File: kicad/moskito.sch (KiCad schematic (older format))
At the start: 0 parts

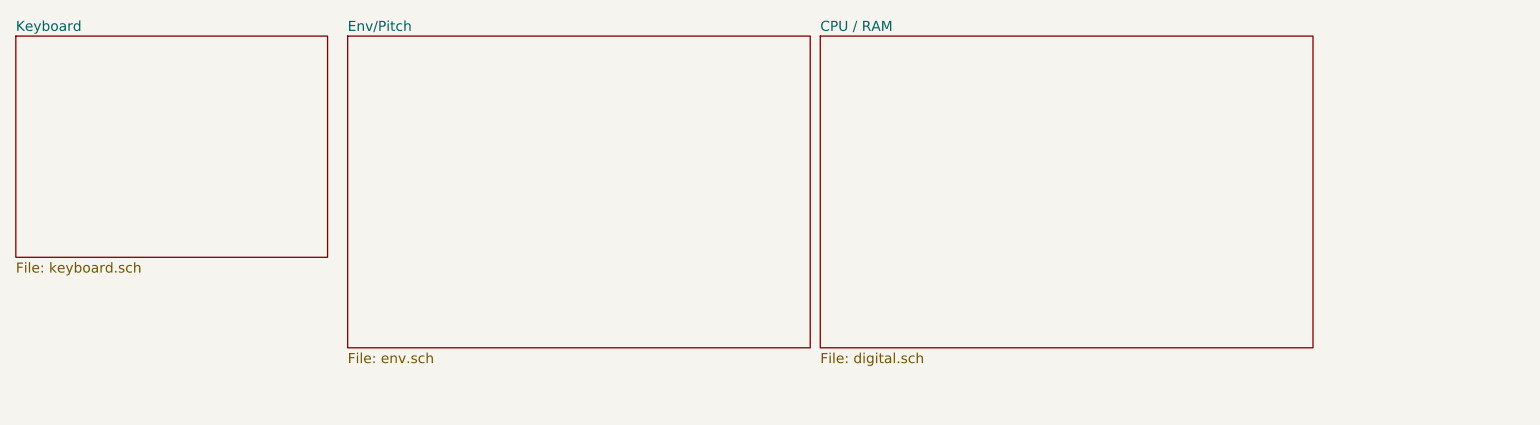
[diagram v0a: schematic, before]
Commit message: 'a'
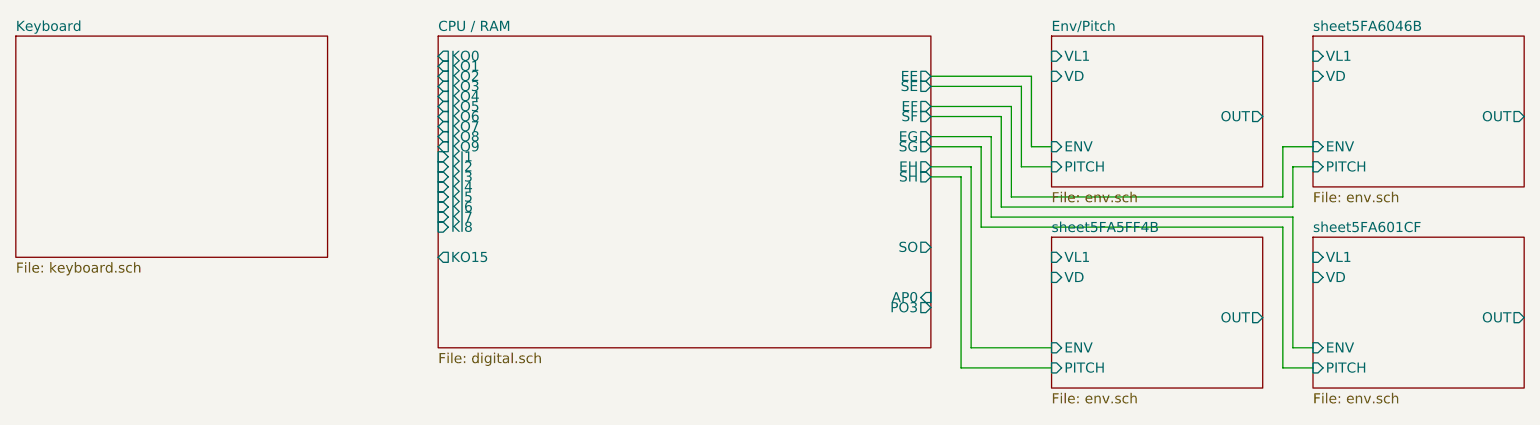
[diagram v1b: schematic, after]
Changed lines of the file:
@@
 $Descr A4 11693 8268
 encoding utf-8
-Sheet 1 4
+Sheet 1 7
 Title ""
 Date ""
@@
 $EndSheet
 $Sheet
-S 2350 700  2300 1550
+S 5850 700  1050 750
 U 5F3D82C3
 F0 "Env/Pitch" 50
 F1 "env.sch" 50
+F2 "ENV" I L 5850 1250 50
+F3 "PITCH" I L 5850 1350 50
+F4 "VD" I L 5850 900 50
+F5 "VL1" I L 5850 800 50
+F6 "OUT" O R 6900 1100 50
 $EndSheet
 $Sheet
-S 4700 700  2450 1550
+S 2800 700  2450 1550
 U 5F82B739
 F0 "CPU / RAM" 50
 F1 "digital.sch" 50
+F2 "KO1" O L 2800 850 50
+F3 "KO2" O L 2800 900 50
+F4 "KO3" O L 2800 950 50
+F5 "KO4" O L 2800 1000 50
+F6 "KO5" O L 2800 1050 50
+F7 "KO6" O L 2800 1100 50
+F8 "KO7" O L 2800 1150 50
+F9 "KO8" O L 2800 1200 50
+F10 "KO9" O L 2800 1250 50
+F11 "KO0" O L 2800 800 50
+F12 "KI1" I L 2800 1300 50
+F13 "KI2" I L 2800 1350 50
+F14 "KI3" I L 2800 1400 50
+F15 "KI4" I L 2800 1450 50
+F16 "KI5" I L 2800 1500 50
+F17 "KI6" I L 2800 1550 50
+F18 "KI7" I L 2800 1600 50
+F19 "KI8" I L 2800 1650 50
+F20 "KO15" O L 2800 1800 50
+F21 "EH" O R 5250 1350 50
+F22 "EG" O R 5250 1200 50
+F23 "EF" O R 5250 1050 50
+F24 "EE" O R 5250 900 50
+F25 "SH" O R 5250 1400 50
+F26 "SG" O R 5250 1250 50
+F27 "SF" O R 5250 1100 50
+F28 "SE" O R 5250 950 50
+F29 "SO" O R 5250 1750 50
+F30 "PO3" O R 5250 2050 50
+F31 "AP0" I R 5250 2000 50
 $EndSheet
+$Sheet
+S 5850 1700 1050 750
+U 5FA5FF52
+F0 "sheet5FA5FF4B" 50
+F1 "env.sch" 50
+F2 "ENV" I L 5850 2250 50
+F3 "PITCH" I L 5850 2350 50
+F4 "VD" I L 5850 1900 50
+F5 "VL1" I L 5850 1800 50
+F6 "OUT" O R 6900 2100 50
+$EndSheet
+$Sheet
+S 7150 1700 1050 750
+U 5FA601D6
+F0 "sheet5FA601CF" 50
+F1 "env.sch" 50
+F2 "ENV" I L 7150 2250 50
+F3 "PITCH" I L 7150 2350 50
+F4 "VD" I L 7150 1900 50
+F5 "VL1" I L 7150 1800 50
+F6 "OUT" O R 8200 2100 50
+$EndSheet
+$Sheet
+S 7150 700  1050 750
+U 5FA60472
+F0 "sheet5FA6046B" 50
+F1 "env.sch" 50
+F2 "ENV" I L 7150 1250 50
+F3 "PITCH" I L 7150 1350 50
+F4 "VD" I L 7150 900 50
+F5 "VL1" I L 7150 800 50
+F6 "OUT" O R 8200 1100 50
+$EndSheet
+Wire Wire Line
+	5250 1400 5400 1400
+Wire Wire Line
+	5400 2350 5850 2350
+Wire Wire Line
+	5850 1350 5700 1350
+Wire Wire Line
+	5700 1350 5700 950
+Wire Wire Line
+	5700 950  5250 950
+Wire Wire Line
+	5850 1250 5750 1250
+Wire Wire Line
+	5750 1250 5750 900
+Wire Wire Line
+	5750 900  5250 900
+Wire Wire Line
+	5400 1400 5400 2350
+Wire Wire Line
+	5450 1350 5250 1350
+Wire Wire Line
+	5850 2250 5450 2250
+Wire Wire Line
+	5450 2250 5450 1350
+Wire Wire Line
+	5250 1250 5500 1250
+Wire Wire Line
+	5500 1250 5500 1650
+Wire Wire Line
+	5500 1650 7000 1650
+Wire Wire Line
+	7000 1650 7000 2350
+Wire Wire Line
+	7000 2350 7150 2350
+Wire Wire Line
+	7150 2250 7050 2250
+Wire Wire Line
+	7050 2250 7050 1600
+Wire Wire Line
+	7050 1600 5550 1600
+Wire Wire Line
+	5550 1200 5250 1200
+Wire Wire Line
+	5550 1200 5550 1600
+Wire Wire Line
+	7150 1350 7050 1350
+Wire Wire Line
+	7050 1350 7050 1550
+Wire Wire Line
+	7050 1550 5600 1550
+Wire Wire Line
+	5600 1550 5600 1100
+Wire Wire Line
+	5600 1100 5250 1100
+Wire Wire Line
+	5250 1050 5650 1050
+Wire Wire Line
+	5650 1050 5650 1500
+Wire Wire Line
+	5650 1500 7000 1500
+Wire Wire Line
+	7000 1500 7000 1250
+Wire Wire Line
+	7000 1250 7150 1250
 $EndSCHEMATC
